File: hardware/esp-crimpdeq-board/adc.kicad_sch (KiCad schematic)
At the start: 13 parts, among them IC1 ADS1235IRHBT, IC3 ADS1230IPWR

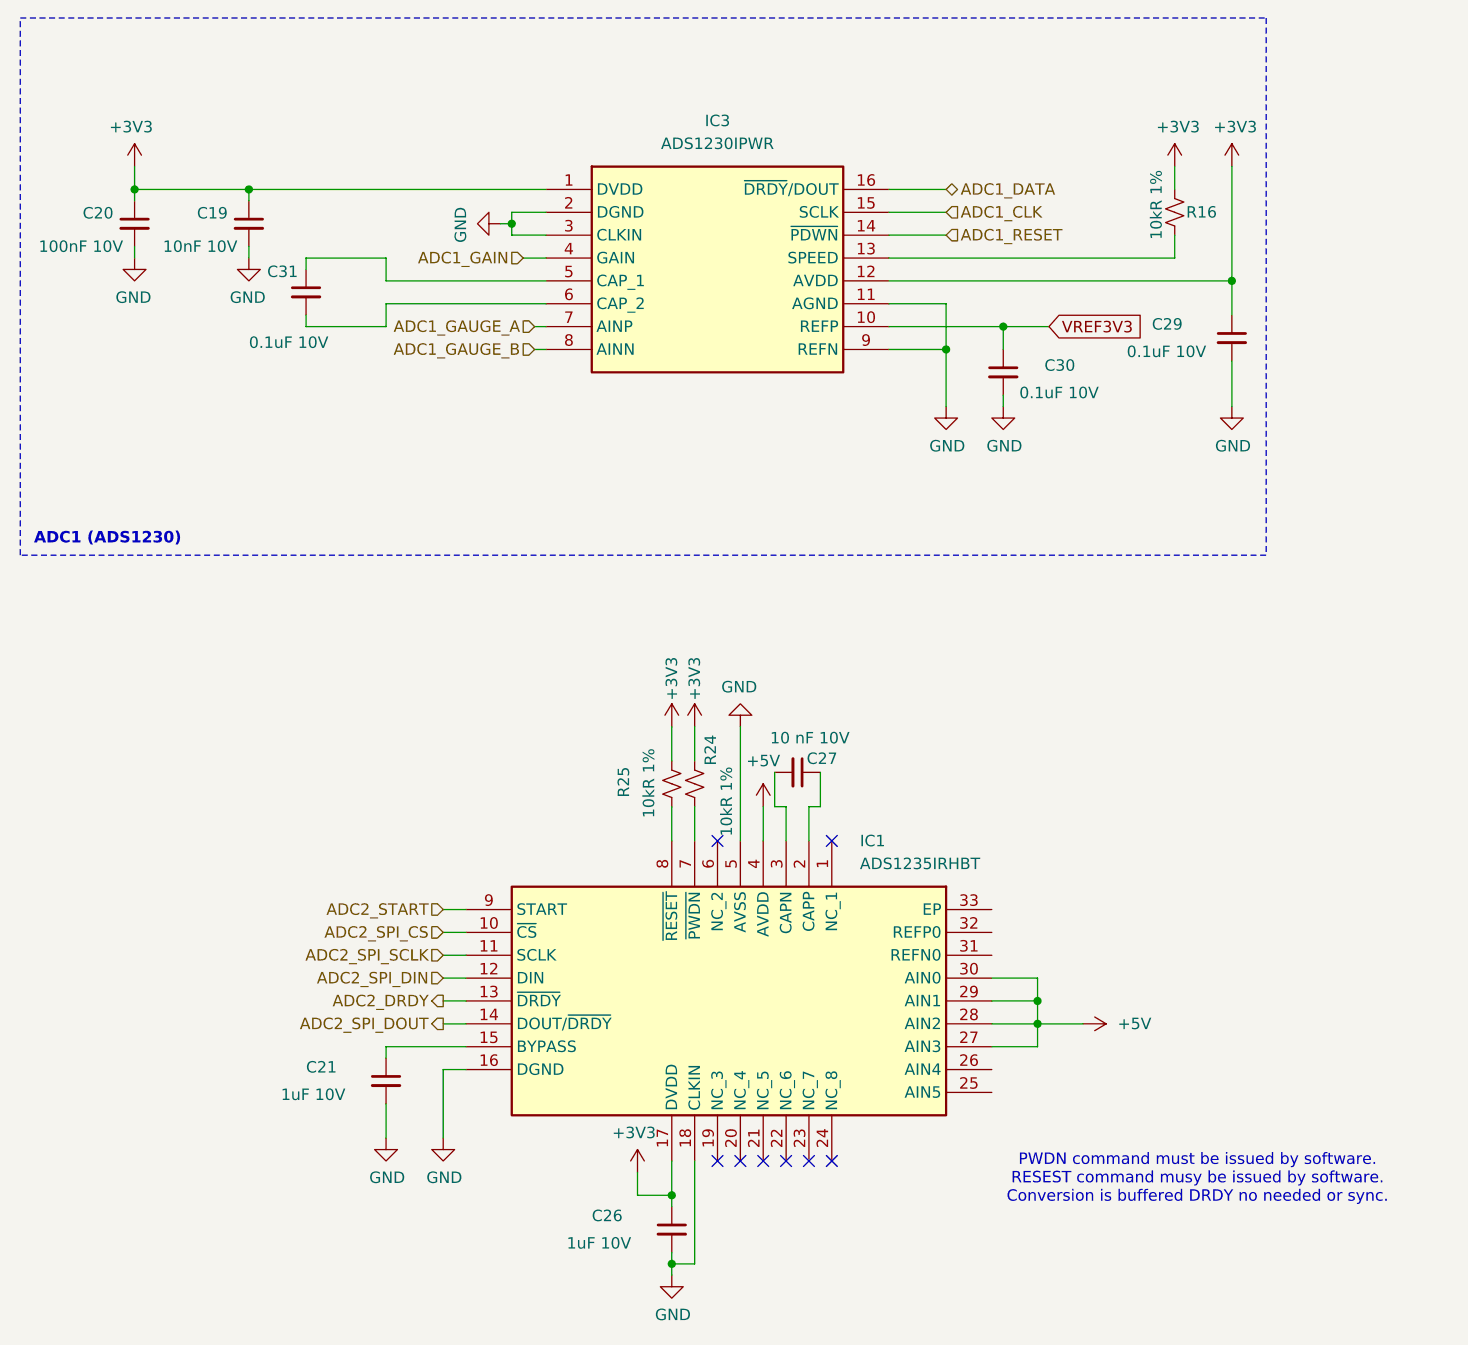
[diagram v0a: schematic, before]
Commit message: feat: Organice schematic
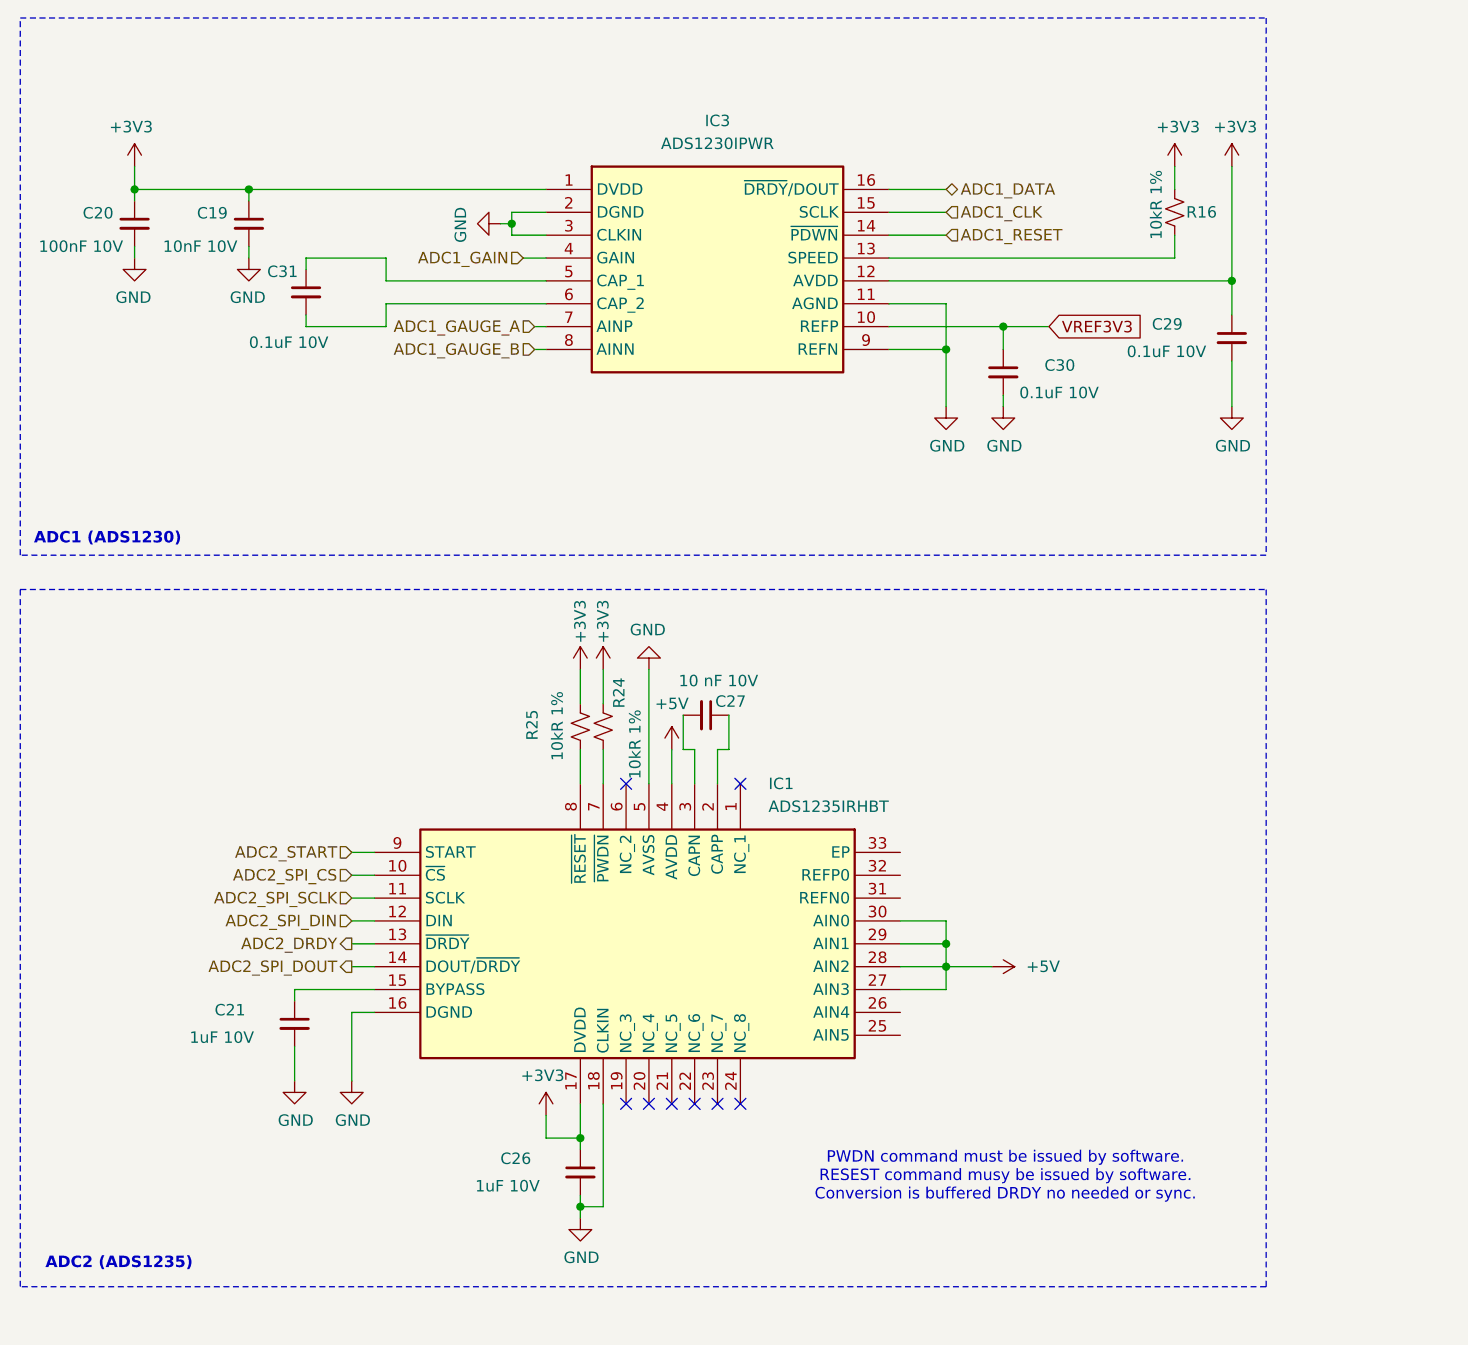
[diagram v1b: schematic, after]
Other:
- note added: "ADC2 (ADS1235)"
- moved on the sheet: C21, C26, C27, IC1, R24, R25
